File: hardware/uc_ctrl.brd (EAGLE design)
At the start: 30 x 33 mm, 31 parts, among them Q4 si2305cd, Q7 si2305cd, T1 BC846, T3 BC846, Y1 32768Hz CFPX-217 12.5pF

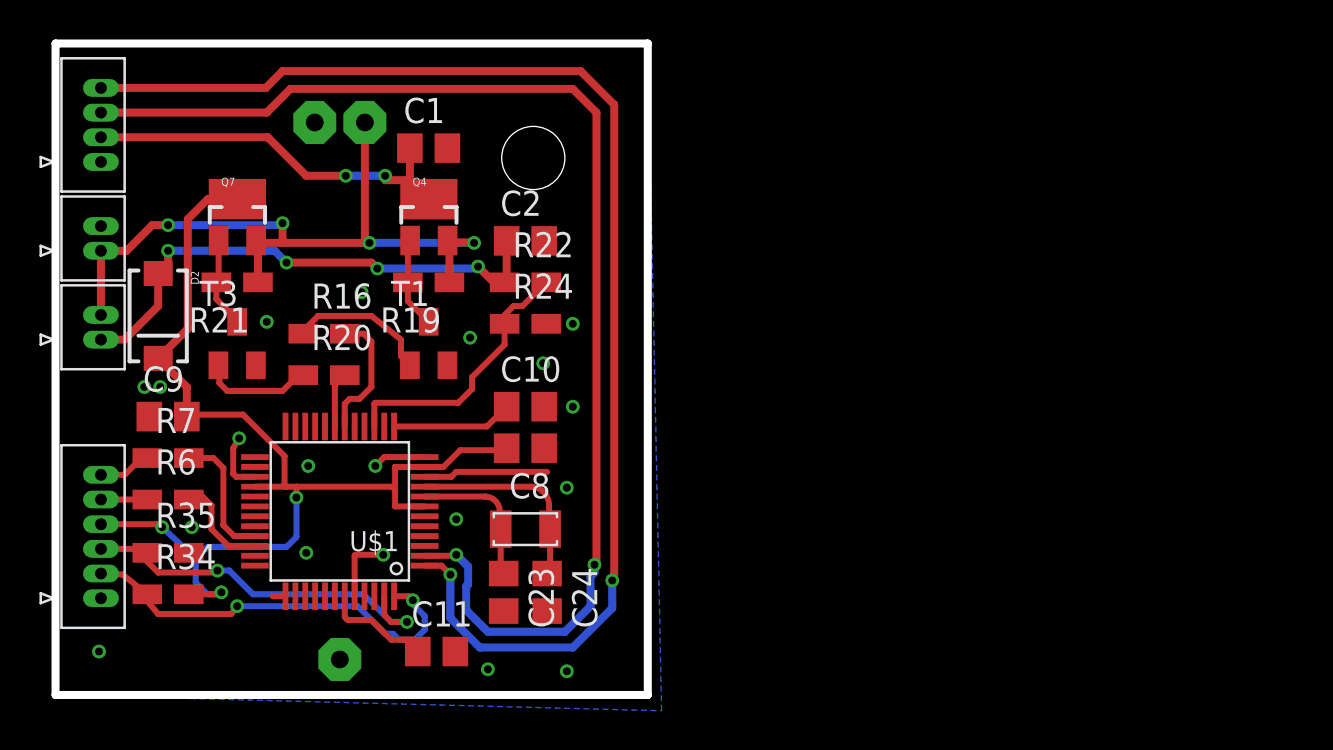
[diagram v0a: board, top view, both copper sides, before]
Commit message: rev 2
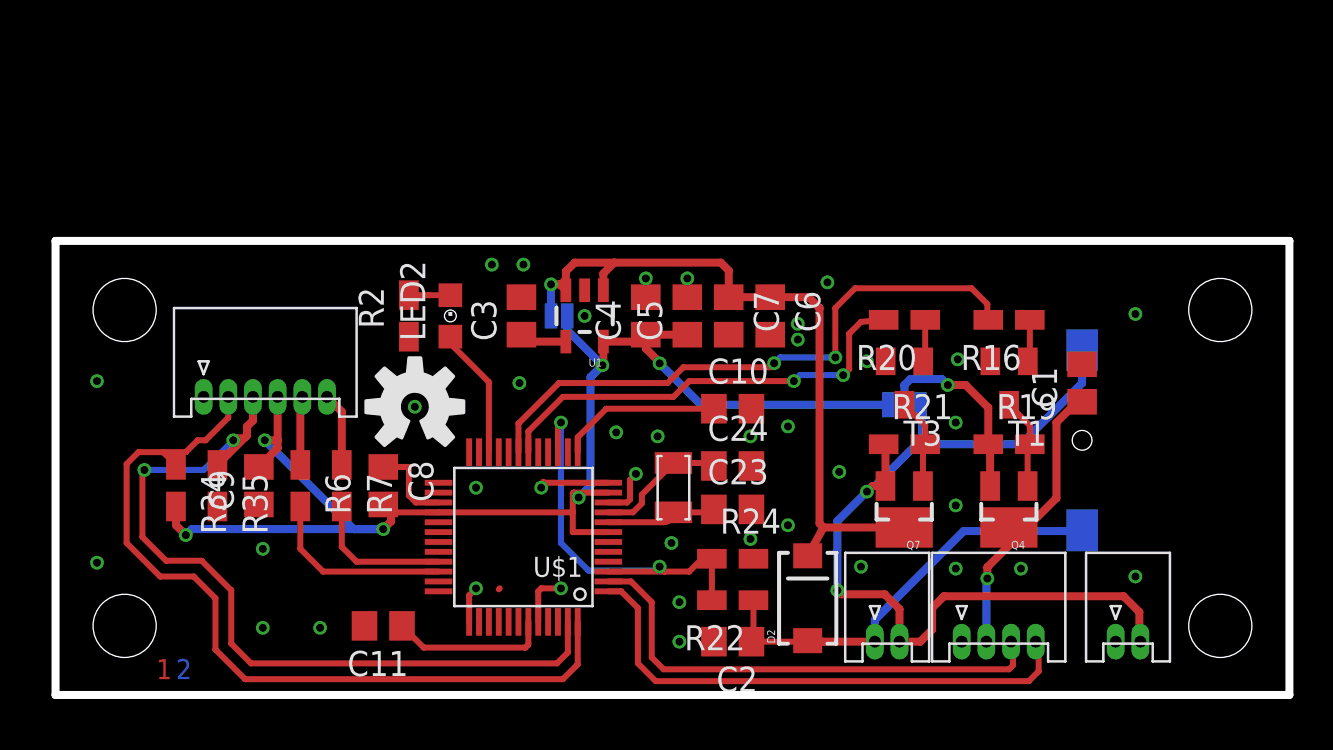
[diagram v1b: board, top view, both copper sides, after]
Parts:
- removed G1: HU2032-LF, Simplex-Battery:HU2032-LF
- removed U$9: push_button, Simplex-Connectors:0530470210
- added C3, C4, C7: 100nF, rcl:C0805
- added C5, C6: 10uF, rcl:C0805
- added LED2: green, led:CHIPLED_0805
- added R2: 100k, rcl:R0805W
- added SJ1: (no value), SparkFun-Passives:SJ_3_PASTE1&2
- added SJ2: SOLDERJUMPERNC2, SparkFun-Passives:SJ_2S-NOTRACE
- added U$4: SPST_TACTILE_SW, Simplex-Switches:6X3.5_TACTILE_SW
- added U$6: MOLEX_2HORIZONTAL, Simplex-Connectors:0530480210
- added U1: 3vLDO, SparkFun-PowerIC:SOT23-5
- U$2: device Simplex-Connectors:0530470610 -> Simplex-Connectors:0530480610
- U$3: value ucurrent -> MOLEX_4HORIZONTAL; device Simplex-Connectors:0530470410 -> Simplex-Connectors:0530480401
- U$5: value external_pow -> sw; device Simplex-Connectors:0530470210 -> Simplex-Connectors:0530480210
- moved U$3 49.9 mm to (45.9, 2.70), turned to 0 degrees
- moved U$5 43.9 mm to (41.5, 2.70), turned to 0 degrees
- moved Q7 37.1 mm to (43.0, 9.20), turned to 180 degrees
- moved D2 35.9 mm to (38.1, 4.90), turned to 90 degrees
- moved C1 35.2 mm to (52.0, 15.8), turned to 90 degrees
- moved R21 34.8 mm to (43.0, 12.7), turned to 0 degrees
- moved R16 34.7 mm to (48.3, 19.0), turned to 180 degrees
- moved T3 33.9 mm to (43.0, 15.8), turned to 180 degrees
- moved Q4 33.1 mm to (48.3, 9.20), turned to 180 degrees
- moved R19 30.5 mm to (48.3, 12.7), turned to 0 degrees
- moved R20 29.5 mm to (43.0, 19.0), turned to 180 degrees
- moved T1 29.5 mm to (48.3, 15.8), turned to 180 degrees
- moved C2 22.9 mm to (34.3, 2.70), turned to 180 degrees
- moved R22 19.2 mm to (34.3, 4.80), turned to 180 degrees
- moved R24 15.9 mm to (34.3, 6.90)
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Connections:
- net P6.0 renamed VREF
- net P6.1 renamed VOUT
- removed net 3V_CELL: G1.+, Q4.2, Q7.2, R19.1, R21.1, U$5.1, U$9.2
- removed net P1.1: R22.2, R24.1, U$1.15
- new net N$1: LED2.C, R2.2
- new net N$2: LED2.A, U$1.22
- new net N$4: C6.1, C7.1, D2.C, Q7.3, SJ2.1, U1.1, U1.3
- new net N$5: C3.1, U1.4
- new net N$8: Q4.2, R19.1, SJ1.2
- new net VBAT: R22.2, R24.1, U$1.15, U$1.3
- new net VCC_IN: Q7.2, R21.1, SJ1.3, U$4.1, U$5.P$2, U$6.P$2
- net GND: now also C3.2, C4.2, C5.2, C6.2, C7.2, R2.1, U$6.P$1, U1.2; no longer G1.-, U$5.2
- net PUSH: now also U$4.2, U$5.P$1; no longer U$9.1
- net UC_EN: now also U$1.19; no longer U$1.18
- net VCC: now also C4.1, C5.1, SJ1.1, SJ2.2, U1.5; no longer D2.C, Q7.3
- net VCC_EN: now also U$1.18; no longer U$1.19
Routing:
- net VCC_IN: track 0.00 -> 46.5 mm, vias 0 -> 2
- net VREF: track 65.9 -> 27.0 mm, vias 2 -> 0
- net VOUT: track 63.2 -> 25.3 mm, vias 2 -> 0
- net 3V_CELL: track 36.9 -> 0.00 mm, vias 4 -> 0
- net N$4: track 0.00 -> 36.8 mm, vias 0 -> 1
- net UC_EN: track 6.67 -> 30.7 mm, vias 0 -> 2
- net VBAT: track 0.00 -> 21.5 mm, vias 0 -> 2
- net TEST: track 19.9 -> 41.1 mm
- net RST: track 21.3 -> 41.8 mm, vias 2 -> 0
- net VCC_EN: track 2.81 -> 22.4 mm, vias 0 -> 2
- net VCC: track 56.4 -> 71.2 mm, vias 3 -> 6
- net P1.1: track 13.8 -> 0.00 mm
- net N$8: track 0.00 -> 10.0 mm, vias 0 -> 1
- net N$2: track 0.00 -> 6.66 mm
- net N$3: track 7.32 -> 2.12 mm
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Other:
- board size 30 x 33 mm -> 62.5 x 23 mm
- board text added: "1"
- board text added: "2"
- board text added: "SJ1"
- board text added: "SJ2"
- board text added: "VBAT+ out"
- board text added: "VBAT- out"
- board text added: "Vcc_in"
- board text added: "Vout+ in"
- board text added: "Vout- in"
- board text added: "battery"
- board text added: "debug"
- board text added: "ext_sw"
- board text added: "if Vcc_in is between 2.8-3.0 V SJ1 - short open SJ2 - short if Vcc_in is between 3.1-5.0V SJ1 - open short SJ2 - open"
- board text added: "rev 2.0 201312"
- board text removed: "3V"
- board text removed: "Vcc"
- board text removed: "Vout"
- board text removed: "Vref"
- board text removed: "rev 1.0 201312"
- board text removed: "sw"
